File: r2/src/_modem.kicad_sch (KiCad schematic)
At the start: 37 parts, among them J1 , J11 SMA, J12 U_FL-R-SMT-1_10_, J13 JAE_SIM_Card_SF72S006, J2 , J3 , J4 , J5 , J6 , J7 , J8 , J9 , T10 , T11 , T8 , T9 , U7 Sierra_Wireless_RC7620, U8 ESD7004, U9 TXS0108EPW

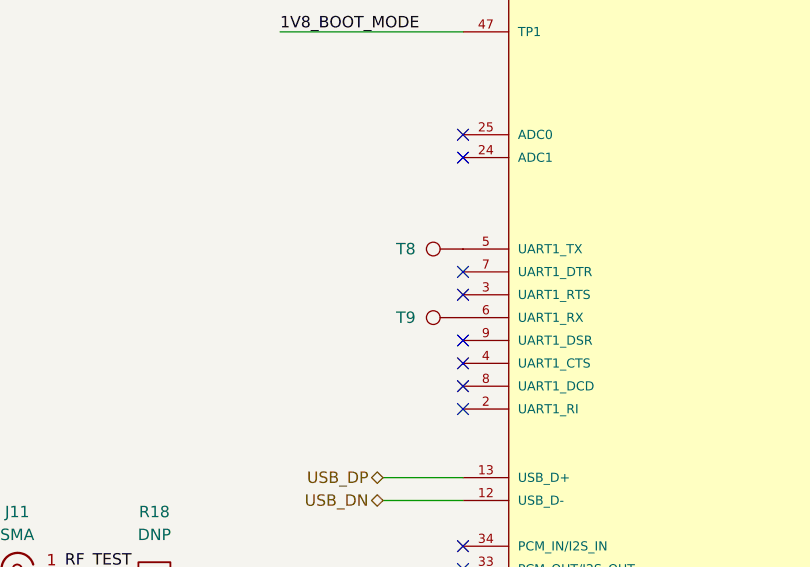
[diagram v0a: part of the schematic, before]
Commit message: Loads of weird library bollocks resolved.
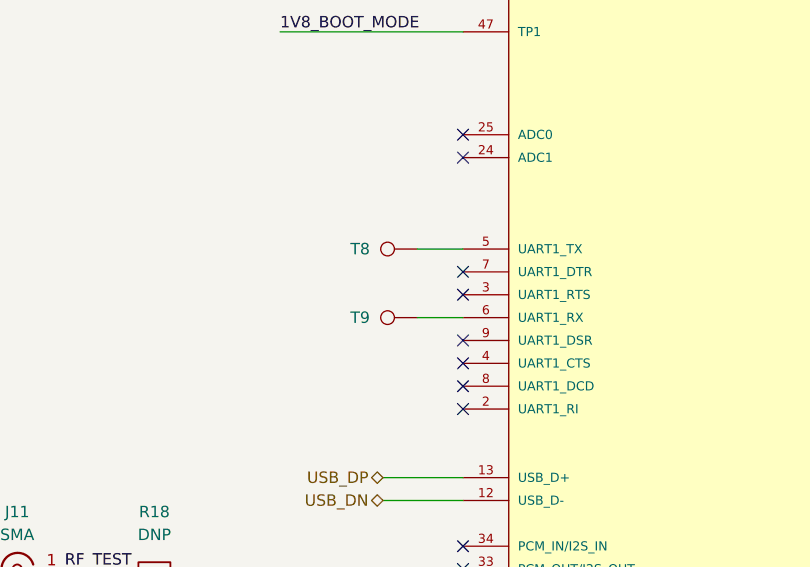
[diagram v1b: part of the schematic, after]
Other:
- moved on the sheet: T8, T9
